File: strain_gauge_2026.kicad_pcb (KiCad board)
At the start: 2 copper layers, 22 parts, among them J2 Conn_01x04_Socket, J3 Conn_01x04_Socket, J5 Conn_01x04_Socket, U1 NAU7802SGI

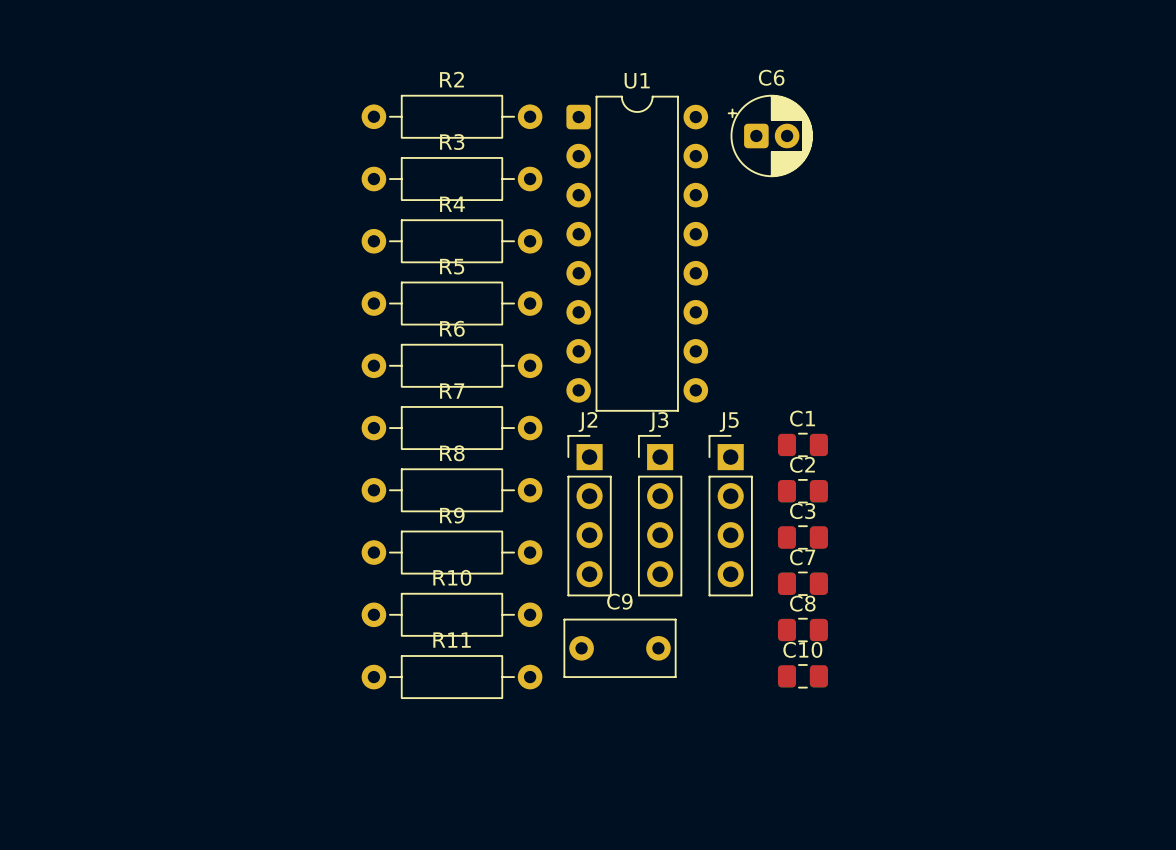
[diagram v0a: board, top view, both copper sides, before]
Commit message: Initial PCB Layout
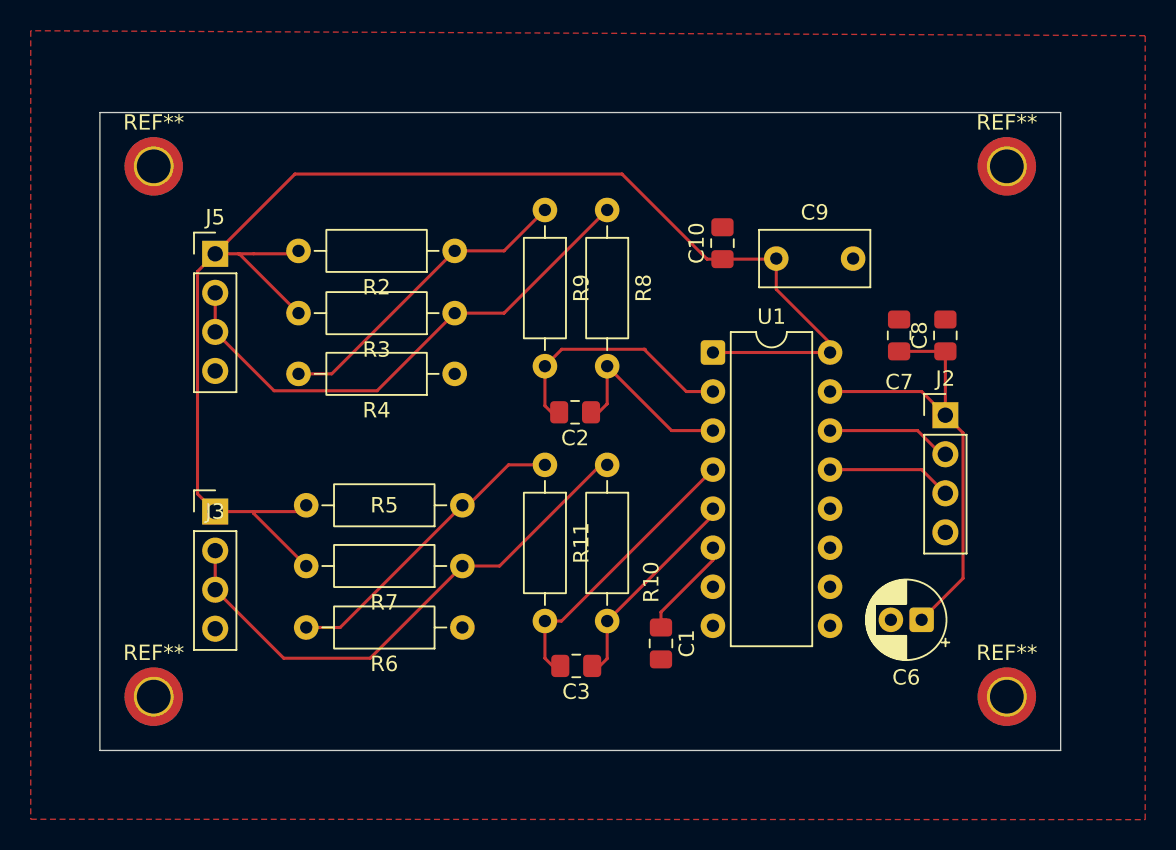
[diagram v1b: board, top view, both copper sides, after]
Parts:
- added REF**: MountingHole_2.2mm_M2_DIN965_Pad_TopBottom, MountingHole:MountingHole_2.2mm_M2_DIN965_Pad_TopBottom, F.Cu at (173.0, 116.0)
- added REF**: MountingHole_2.2mm_M2_DIN965_Pad_TopBottom, MountingHole:MountingHole_2.2mm_M2_DIN965_Pad_TopBottom, F.Cu at (117.5, 116.0)
- added REF**: MountingHole_2.2mm_M2_DIN965_Pad_TopBottom, MountingHole:MountingHole_2.2mm_M2_DIN965_Pad_TopBottom, F.Cu at (117.5, 81.5)
- added REF**: MountingHole_2.2mm_M2_DIN965_Pad_TopBottom, MountingHole:MountingHole_2.2mm_M2_DIN965_Pad_TopBottom, F.Cu at (173.0, 81.5)
- moved J5 36.0 mm to (121.5, 87.2)
- moved C6 33.3 mm to (167.5, 111.0), turned to 180 degrees
- moved J3 29.2 mm to (121.5, 104.0)
- moved C10 28.7 mm to (154.5, 86.5), turned to 90 degrees
- moved C9 28.3 mm to (158.0, 87.5)
- moved R9 24.9 mm to (142.9, 84.3), turned to -90 degrees
- moved R8 23.7 mm to (147.0, 84.3), turned to -90 degrees
- moved J2 23.3 mm to (169.0, 97.7)
- moved C8 21.3 mm to (169.0, 92.5), turned to 90 degrees
- moved R10 18.0 mm to (147.0, 100.9), turned to -90 degrees
- moved R6 18.0 mm to (137.6, 111.5), turned to 180 degrees
- moved R11 17.7 mm to (142.9, 100.9), turned to -90 degrees
- moved U1 17.6 mm to (153.9, 93.6)
- moved C7 17.3 mm to (166.0, 92.5), turned to 90 degrees
- moved C3 16.9 mm to (145.0, 114.0), turned to 180 degrees
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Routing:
- net V_excitation: track 0.00 -> 96.8 mm
- net B+: track 0.00 -> 35.1 mm
- net A+: track 0.00 -> 34.5 mm
- net +3V3: track 0.00 -> 30.6 mm
- net A-: track 0.00 -> 20.4 mm
- net B-: track 0.00 -> 20.4 mm
- net Net-(U1-VIN2N): track 0.00 -> 18.8 mm
- net Net-(U1-VIN1N): track 0.00 -> 16.5 mm
- net Net-(U1-VIN2P): track 0.00 -> 14.0 mm
- net Net-(U1-VIN1P): track 0.00 -> 12.6 mm
- net SDA_MCU: track 0.00 -> 8.29 mm
- net SCLK_MCU: track 0.00 -> 8.29 mm
- net Net-(U1-VBG): track 0.00 -> 6.43 mm
- added copper zone on F.Cu, net GND
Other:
- board outline added: 62.5 x 41.5 mm
